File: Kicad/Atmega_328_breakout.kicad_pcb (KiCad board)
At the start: 2 copper layers, 73.8 x 62 mm, 71 parts, among them J1 Jack-DC, J10 Conn_01x06, J11 01x03, J12 01x03, J13 01x03, J14 01x03, J15 01x03, J16 01x03, J17 01x03, J18 01x03, J19 Power_connector, J2 01x03, J20 ADC_Connector, J21 PORB++_connector, J22 PORD_connector, J23 Conn_01x01, J24 Device_Connector, J25 Pin out, J26 Com_header, J27 Power terminal, J28 USB, J3 01x03, J4 01x03, J5 01x03, J6 01x03, J7 01x03, J8 01x03, J9 01x03, Q1 AO3401A, SW1 SW_Push, SW2 SW_Push, U1 NCP1117-5, U2 L7805, U3 LM358, U4 ATMEGA328P-AU, U5 MCP1700-33, U6 MCP2221, Y1 Crystal_GND24

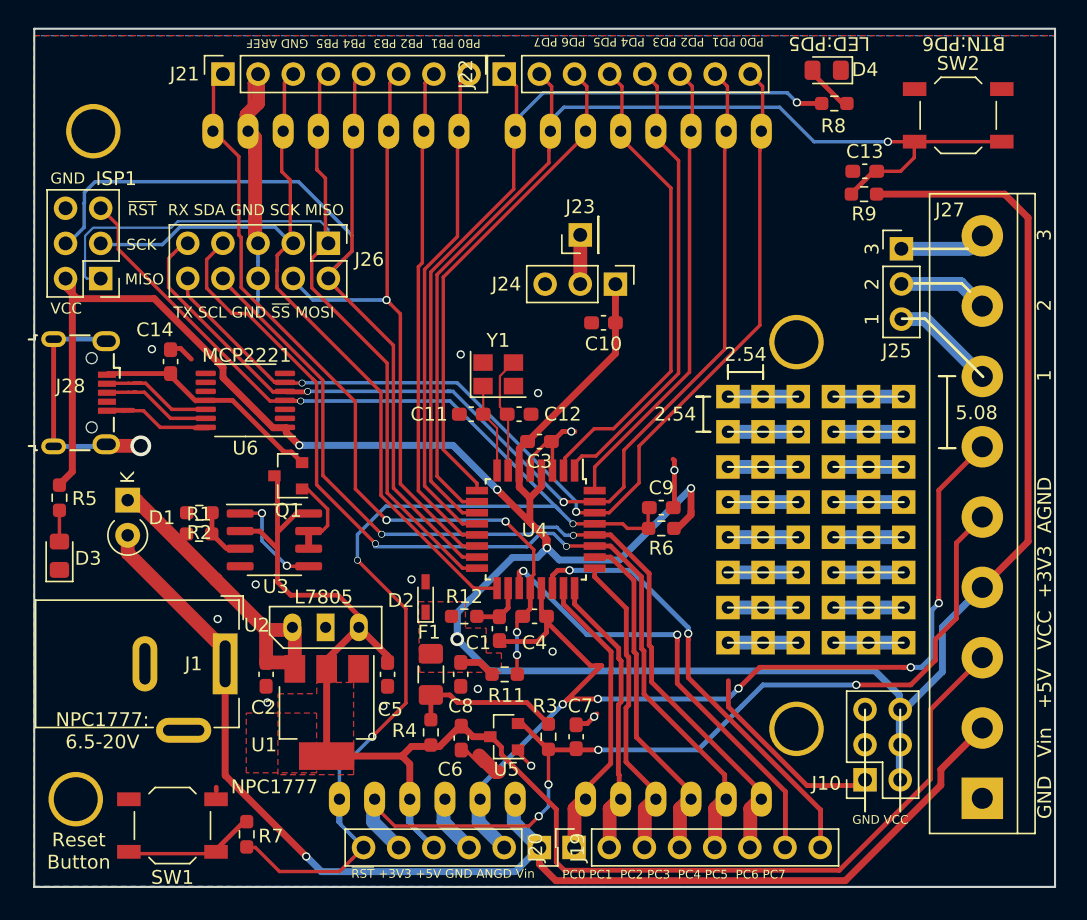
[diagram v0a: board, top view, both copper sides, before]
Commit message: Initial push
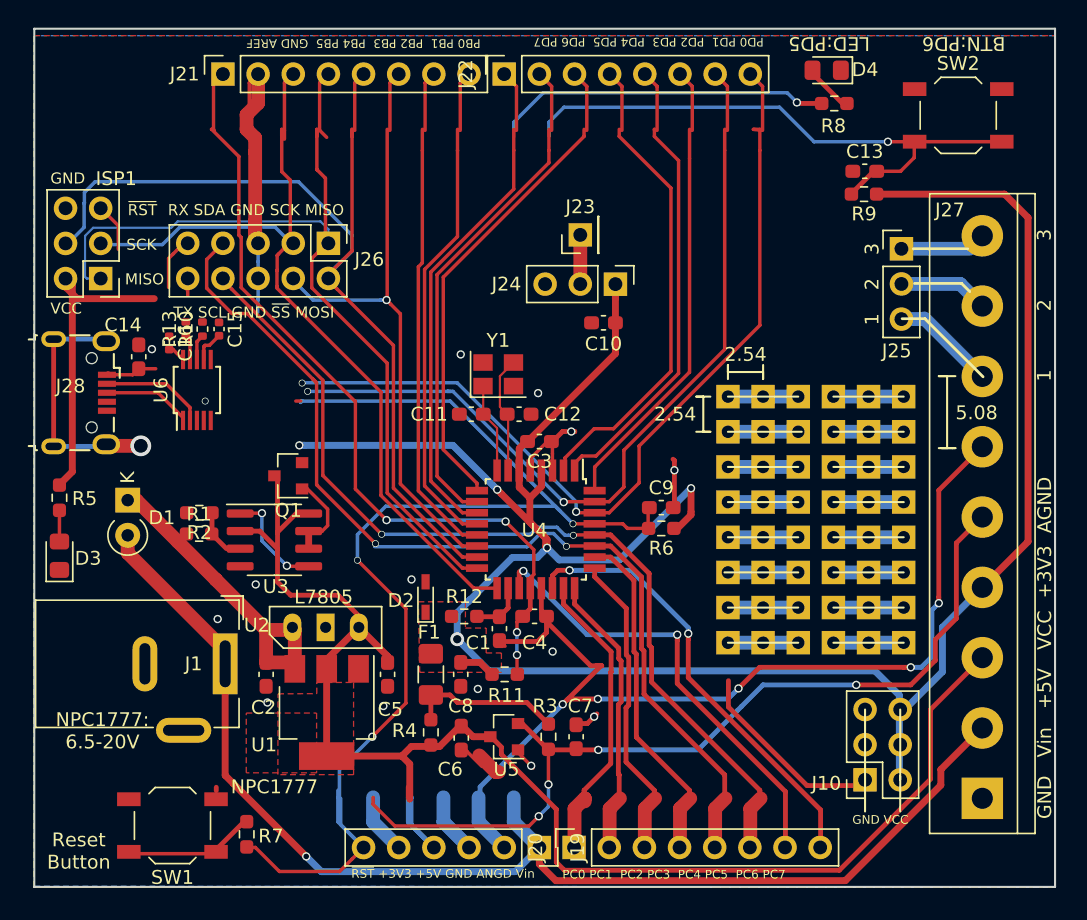
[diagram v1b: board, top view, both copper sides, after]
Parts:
- removed SHIELD1: ATMEL_SHIELD, jorgen:AtmelSHIELD
- added C15: 100n, Capacitor_SMD:C_0402_1005Metric, F.Cu at (63.6, 75.7)
- added C16: 100n, Capacitor_SMD:C_0402_1005Metric, F.Cu at (60.0, 76.7)
- added R10: 120, Resistor_SMD:R_0402_1005Metric, F.Cu at (62.4, 75.7)
- added R13: 120, Resistor_SMD:R_0402_1005Metric, F.Cu at (61.2, 75.7)
- U6: value MCP2221 -> CH340E; footprint Package_SO:TSSOP-14_4.4x5mm_P0.65mm -> Package_SO:MSOP-10_3x3mm_P0.5mm
- moved U6 3.58 mm to (62.0, 80.1), turned to 90 degrees
- moved C14 2.33 mm to (57.8, 77.7)
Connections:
- U6 pad 1: VCC -> Net-(J28-Pad3)
- U6 pad 2: Net-(U6-Pad2) -> Net-(J28-Pad2)
- U6 pad 3: Net-(U6-Pad3) -> GND
- U6 pad 5: PD1(TX) -> Net-(U6-Pad5)
- U6 pad 6: PD0(RX) -> Net-(U6-Pad6)
- U6 pad 7: Net-(U6-Pad7) -> VCC
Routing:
- net ~RESET: track 108.9 -> 91.5 mm, vias 4 -> 3
- net PD1(TX): track 77.1 -> 64.0 mm
- net VCC: track 209.4 -> 196.3 mm
- net VUSB: track 16.2 -> 3.88 mm
- net GND: track 77.6 -> 65.6 mm, vias 14 -> 15
- net PD0(RX): track 78.0 -> 66.5 mm
- net Net-(R10-Pad1): track 0.00 -> 1.86 mm
- net Net-(R13-Pad1): track 0.00 -> 1.81 mm
- net Net-(C16-Pad2): track 0.00 -> 1.30 mm
- net Net-(J28-Pad3): track 7.47 -> 6.45 mm
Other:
- board text removed: "MCP2221"
